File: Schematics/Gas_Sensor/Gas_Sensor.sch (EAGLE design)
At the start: 9 parts, among them J1 RJ45, X1 GAS_SENSOR

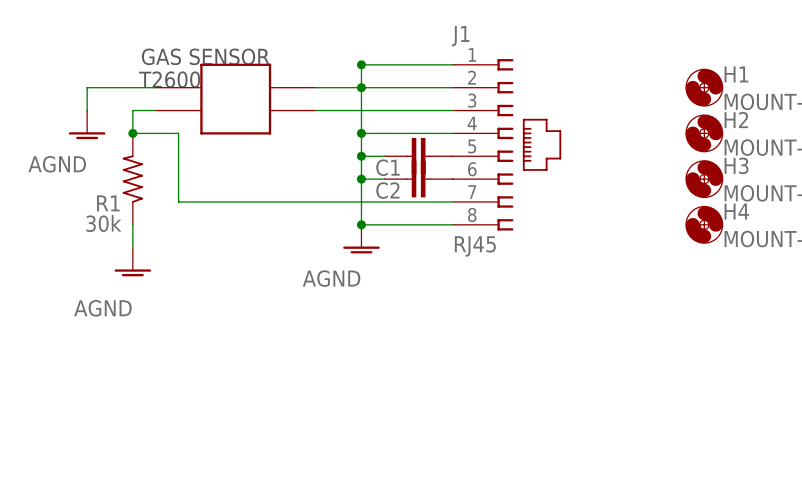
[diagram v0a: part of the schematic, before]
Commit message: Layout for final inspection
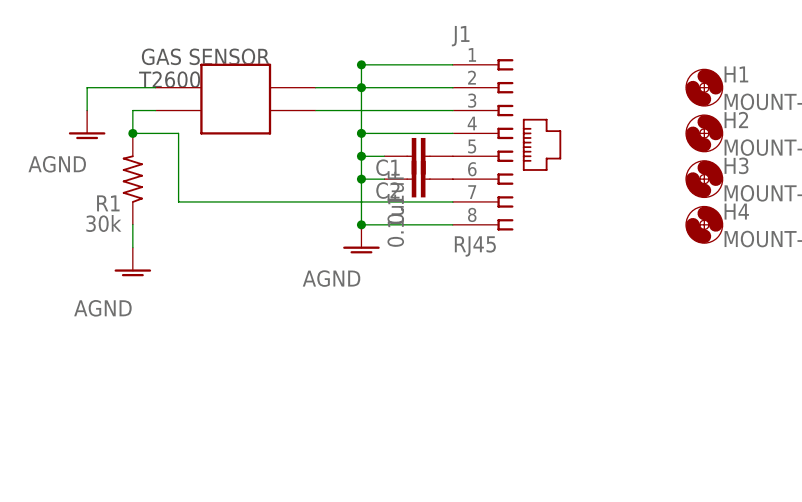
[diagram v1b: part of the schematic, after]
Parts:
- C1, C2: value (none) -> 0.1uF
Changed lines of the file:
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@@
 <?xml version="1.0" encoding="utf-8"?>
 <!DOCTYPE eagle SYSTEM "eagle.dtd">
-<eagle version="6.3">
+<eagle version="6.4">
 <drawing>
 <settings>
@@
 <grid distance="0.1" unitdist="inch" unit="inch" style="lines" multiple="1" display="no" altdistance="0.01" altunitdist="inch" altunit="inch"/>
 <layers>
-<layer number="1" name="Top" color="4" fill="1" visible="yes" active="no"/>
-<layer number="16" name="Bottom" color="1" fill="1" visible="yes" active="no"/>
-<layer number="17" name="Pads" color="2" fill="1" visible="yes" active="no"/>
-<layer number="18" name="Vias" color="2" fill="1" visible="yes" active="no"/>
-<layer number="19" name="Unrouted" color="6" fill="1" visible="yes" active="no"/>
-<layer number="20" name="Dimension" color="15" fill="1" visible="yes" active="no"/>
-<layer number="21" name="tPlace" color="7" fill="1" visible="yes" active="no"/>
-<layer number="22" name="bPlace" color="7" fill="1" visible="yes" active="no"/>
-<layer number="23" name="tOrigins" color="15" fill="1" visible="yes" active="no"/>
-<layer number="24" name="bOrigins" color="15" fill="1" visible="yes" active="no"/>
-<layer number="25" name="tNames" color="7" fill="1" visible="yes" active="no"/>
-<layer number="26" name="bNames" color="7" fill="1" visible="yes" active="no"/>
-<layer number="27" name="tValues" color="7" fill="1" visible="yes" active="no"/>
-<layer number="28" name="bValues" color="7" fill="1" visible="yes" active="no"/>
+<layer number="1" name="Top" color="4" fill="1" visible="no" active="no"/>
+<layer number="16" name="Bottom" color="1" fill="1" visible="no" active="no"/>
+<layer number="17" name="Pads" color="2" fill="1" visible="no" active="no"/>
+<layer number="18" name="Vias" color="2" fill="1" visible="no" active="no"/>
+<layer number="19" name="Unrouted" color="6" fill="1" visible="no" active="no"/>
+<layer number="20" name="Dimension" color="15" fill="1" visible="no" active="no"/>
+<layer number="21" name="tPlace" color="7" fill="1" visible="no" active="no"/>
+<layer number="22" name="bPlace" color="7" fill="1" visible="no" active="no"/>
+<layer number="23" name="tOrigins" color="15" fill="1" visible="no" active="no"/>
+<layer number="24" name="bOrigins" color="15" fill="1" visible="no" active="no"/>
+<layer number="25" name="tNames" color="7" fill="1" visible="no" active="no"/>
+<layer number="26" name="bNames" color="7" fill="1" visible="no" active="no"/>
+<layer number="27" name="tValues" color="7" fill="1" visible="no" active="no"/>
+<layer number="28" name="bValues" color="7" fill="1" visible="no" active="no"/>
 <layer number="29" name="tStop" color="7" fill="3" visible="no" active="no"/>
 <layer number="30" name="bStop" color="7" fill="6" visible="no" active="no"/>
@@
 <layer number="35" name="tGlue" color="7" fill="4" visible="no" active="no"/>
 <layer number="36" name="bGlue" color="7" fill="5" visible="no" active="no"/>
-<layer number="37" name="tTest" color="7" fill="1" visible="yes" active="no"/>
-<layer number="38" name="bTest" color="7" fill="1" visible="yes" active="no"/>
+<layer number="37" name="tTest" color="7" fill="1" visible="no" active="no"/>
+<layer number="38" name="bTest" color="7" fill="1" visible="no" active="no"/>
 <layer number="39" name="tKeepout" color="4" fill="11" visible="no" active="no"/>
 <layer number="40" name="bKeepout" color="1" fill="11" visible="no" active="no"/>
@@
 <layer number="44" name="Drills" color="7" fill="1" visible="no" active="no"/>
 <layer number="45" name="Holes" color="7" fill="1" visible="no" active="no"/>
-<layer number="46" name="Milling" color="3" fill="1" visible="yes" active="no"/>
-<layer number="47" name="Measures" color="7" fill="1" visible="yes" active="no"/>
-<layer number="48" name="Document" color="7" fill="1" visible="yes" active="no"/>
-<layer number="49" name="Reference" color="7" fill="1" visible="yes" active="no"/>
-<layer number="51" name="tDocu" color="7" fill="1" visible="yes" active="no"/>
-<layer number="52" name="bDocu" color="7" fill="1" visible="yes" active="no"/>
+<layer number="46" name="Milling" color="3" fill="1" visible="no" active="no"/>
+<layer number="47" name="Measures" color="7" fill="1" visible="no" active="no"/>
+<layer number="48" name="Document" color="7" fill="1" visible="no" active="no"/>
+<layer number="49" name="Reference" color="7" fill="1" visible="no" active="no"/>
+<layer number="51" name="tDocu" color="7" fill="1" visible="no" active="no"/>
+<layer number="52" name="bDocu" color="7" fill="1" visible="no" active="no"/>
 <layer number="91" name="Nets" color="2" fill="1" visible="yes" active="yes"/>
 <layer number="92" name="Busses" color="1" fill="1" visible="yes" active="yes"/>
@@
 <part name="H2" library="holes" deviceset="MOUNT-HOLE" device="2.8"/>
 <part name="H3" library="holes" deviceset="MOUNT-HOLE" device="2.8"/>
-<part name="C1" library="rcl" deviceset="C-EU" device="C0603K"/>
-<part name="C2" library="rcl" deviceset="C-EU" device="C0603K"/>
+<part name="C1" library="rcl" deviceset="C-EU" device="C0603K" value="0.1uF"/>
+<part name="C2" library="rcl" deviceset="C-EU" device="C0603K" value="0.1uF"/>
 </parts>
 <sheets>
